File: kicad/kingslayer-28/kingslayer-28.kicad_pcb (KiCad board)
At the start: 2 copper layers, 133 x 95 mm, 119 parts, among them IC1 STM32F303CCT7, IC2 IS31FL3731-QFLS2-TR, IC3 LM3940IMP-3.3_NOPB, J1 Conn_01x04_Pin, K1 KEYSW, K10 KEYSW, K11 KEYSW, K12 KEYSW, K13 KEYSW, K14 KEYSW, K15 KEYSW, K16 KEYSW, K17 KEYSW, K18 KEYSW, K19 KEYSW, K2 KEYSW, K20 KEYSW, K21 KEYSW, K22 KEYSW, K24 KEYSW, K25 KEYSW, K26 KEYSW, K27 KEYSW, K28 KEYSW, K3 KEYSW, K4 KEYSW, K5 KEYSW, K6 KEYSW, K7 KEYSW, K8 KEYSW, K9 KEYSW, SW1 SS12D07, X1 IC21008.000M30.0EE1B

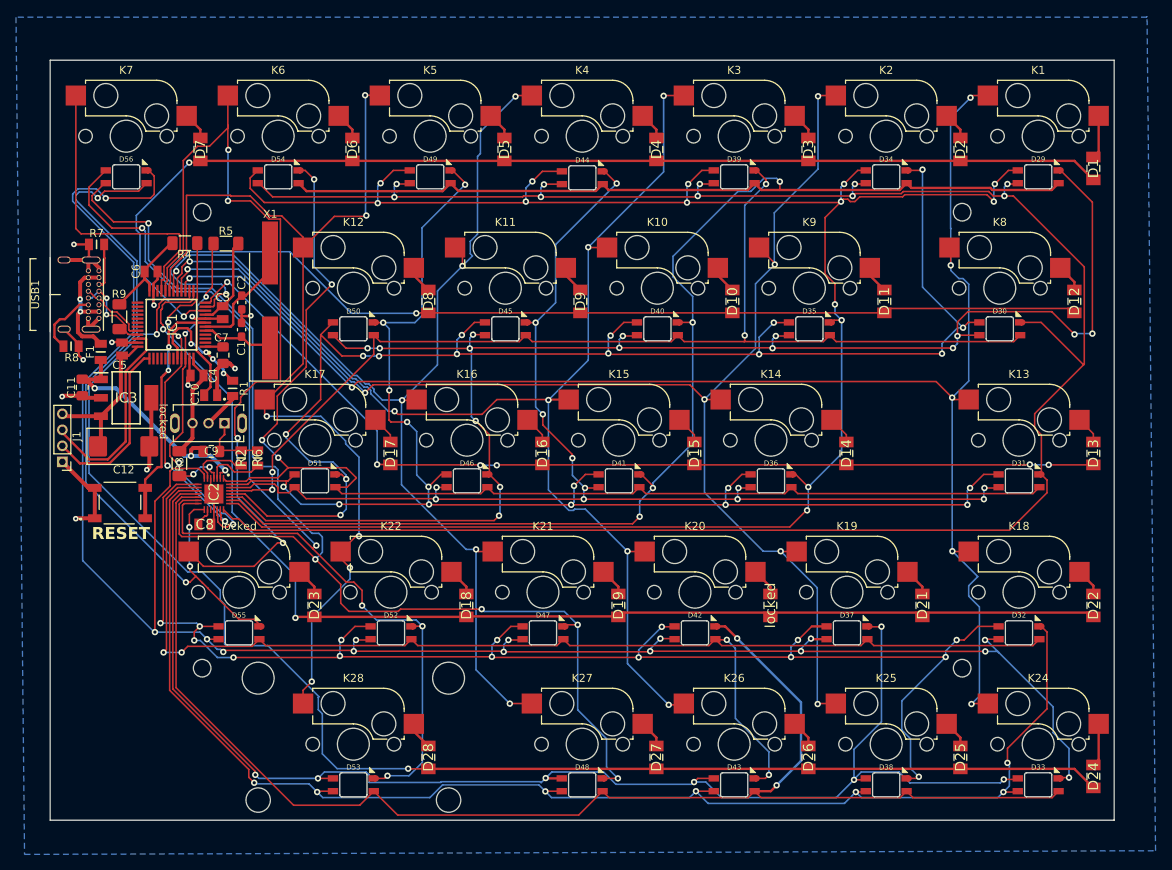
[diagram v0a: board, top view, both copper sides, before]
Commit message: finish DRC
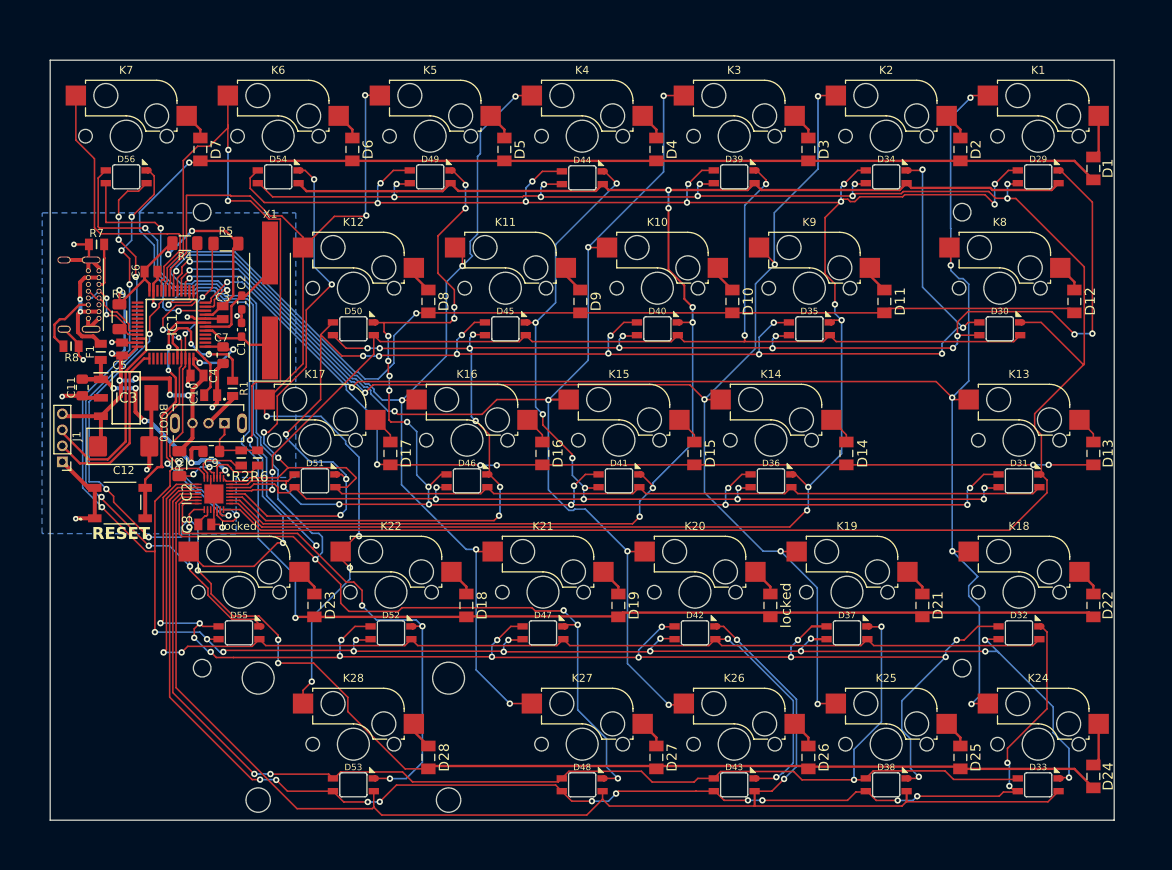
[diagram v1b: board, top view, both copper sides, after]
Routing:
- net +3V3: track 60.2 -> 103.5 mm, vias 0 -> 10
- net cb1: track 252.6 -> 230.7 mm, vias 15 -> 18
- net ca3: track 210.4 -> 200.2 mm, vias 4 -> 6
- net cb5: track 174.0 -> 164.0 mm, vias 7 -> 4
- net cb9: track 92.1 -> 82.3 mm, vias 4 -> 7
- net row1: track 130.2 -> 139.2 mm
- net row3: track 151.7 -> 158.7 mm
- net cb4: track 174.5 -> 168.0 mm, vias 7 -> 12
- net cb6: track 176.9 -> 183.1 mm
- net ca8: track 170.8 -> 175.1 mm, vias 14 -> 19
- net cb3: track 159.6 -> 163.6 mm
- net cb8: track 131.3 -> 134.1 mm
- net row4: track 180.5 -> 182.6 mm, vias 2 -> 6
- net GND: track 83.9 -> 85.9 mm, vias 11 -> 12
- net +5V: track 32.2 -> 34.0 mm, vias 3 -> 5
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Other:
- board text added: "BOOT0"
- board text removed: "locked"
